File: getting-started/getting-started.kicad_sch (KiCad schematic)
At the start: 4 parts, among them SW1 M2011S3A1W03

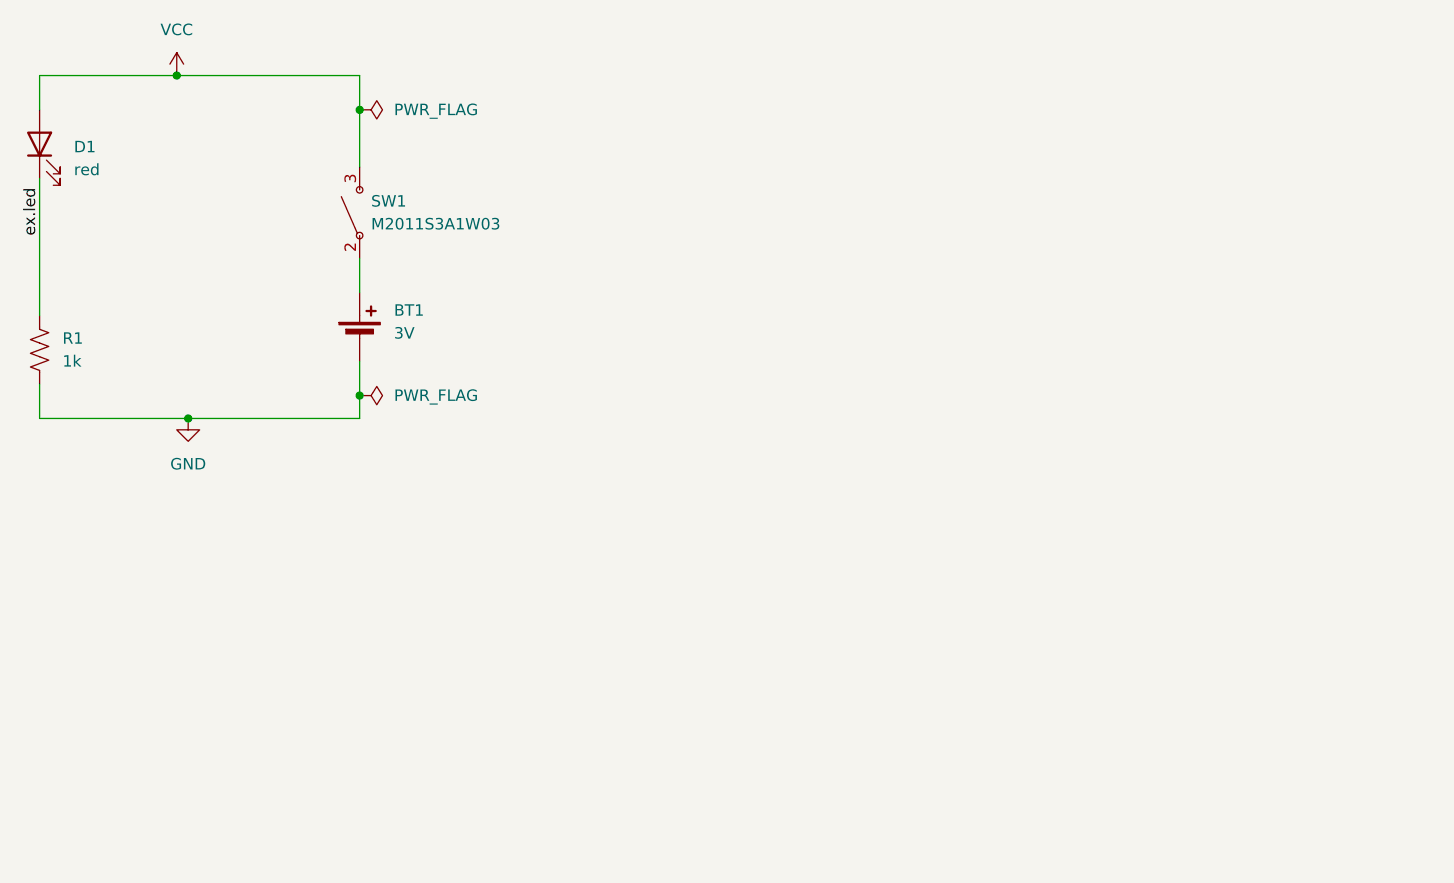
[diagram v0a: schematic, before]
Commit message: 1
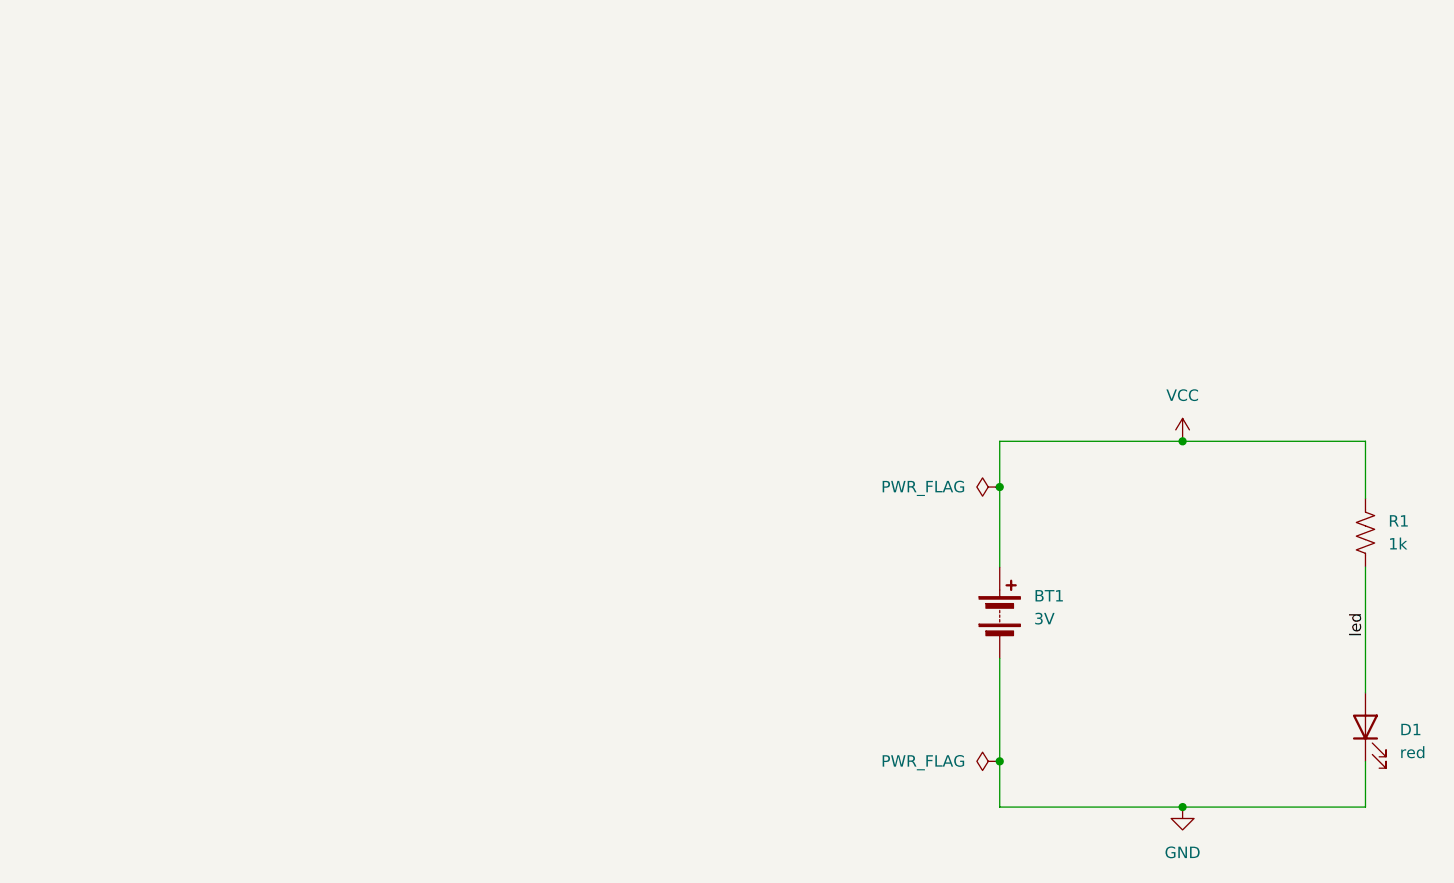
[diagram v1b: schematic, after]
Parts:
- removed BT1: 3V, Battery:BatteryHolder_Keystone_1058_1x2032, symbol Device:Battery_Cell
- removed SW1: M2011S3A1W03, New_Library_0:Switch_Toggle_SPST_NKK_M2011S3A1x03, symbol New_Library_0:M2011S3A1W03
- added BT1: 3V, Battery:BatteryHolder_Keystone_1058_1x2032, symbol Device:Battery
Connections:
- net GND: now also D1.1 (K), BT1.2 (-); no longer R1.2
- net VCC: now also R1.1, BT1.1 (+); no longer D1.2 (A)
- removed net ex.led: D1.1 (K), R1.1
- new net led: D1.2 (A), R1.2
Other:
- title: Led Blank in KiCad 10.0 -> getting-started
